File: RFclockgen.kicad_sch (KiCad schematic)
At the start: 10 parts, among them J1 Conn_01x04_Pin, J3 Conn_01x02_Pin, U2 ESP32-S3-WROOM-1, U3 AP2112K-3.3

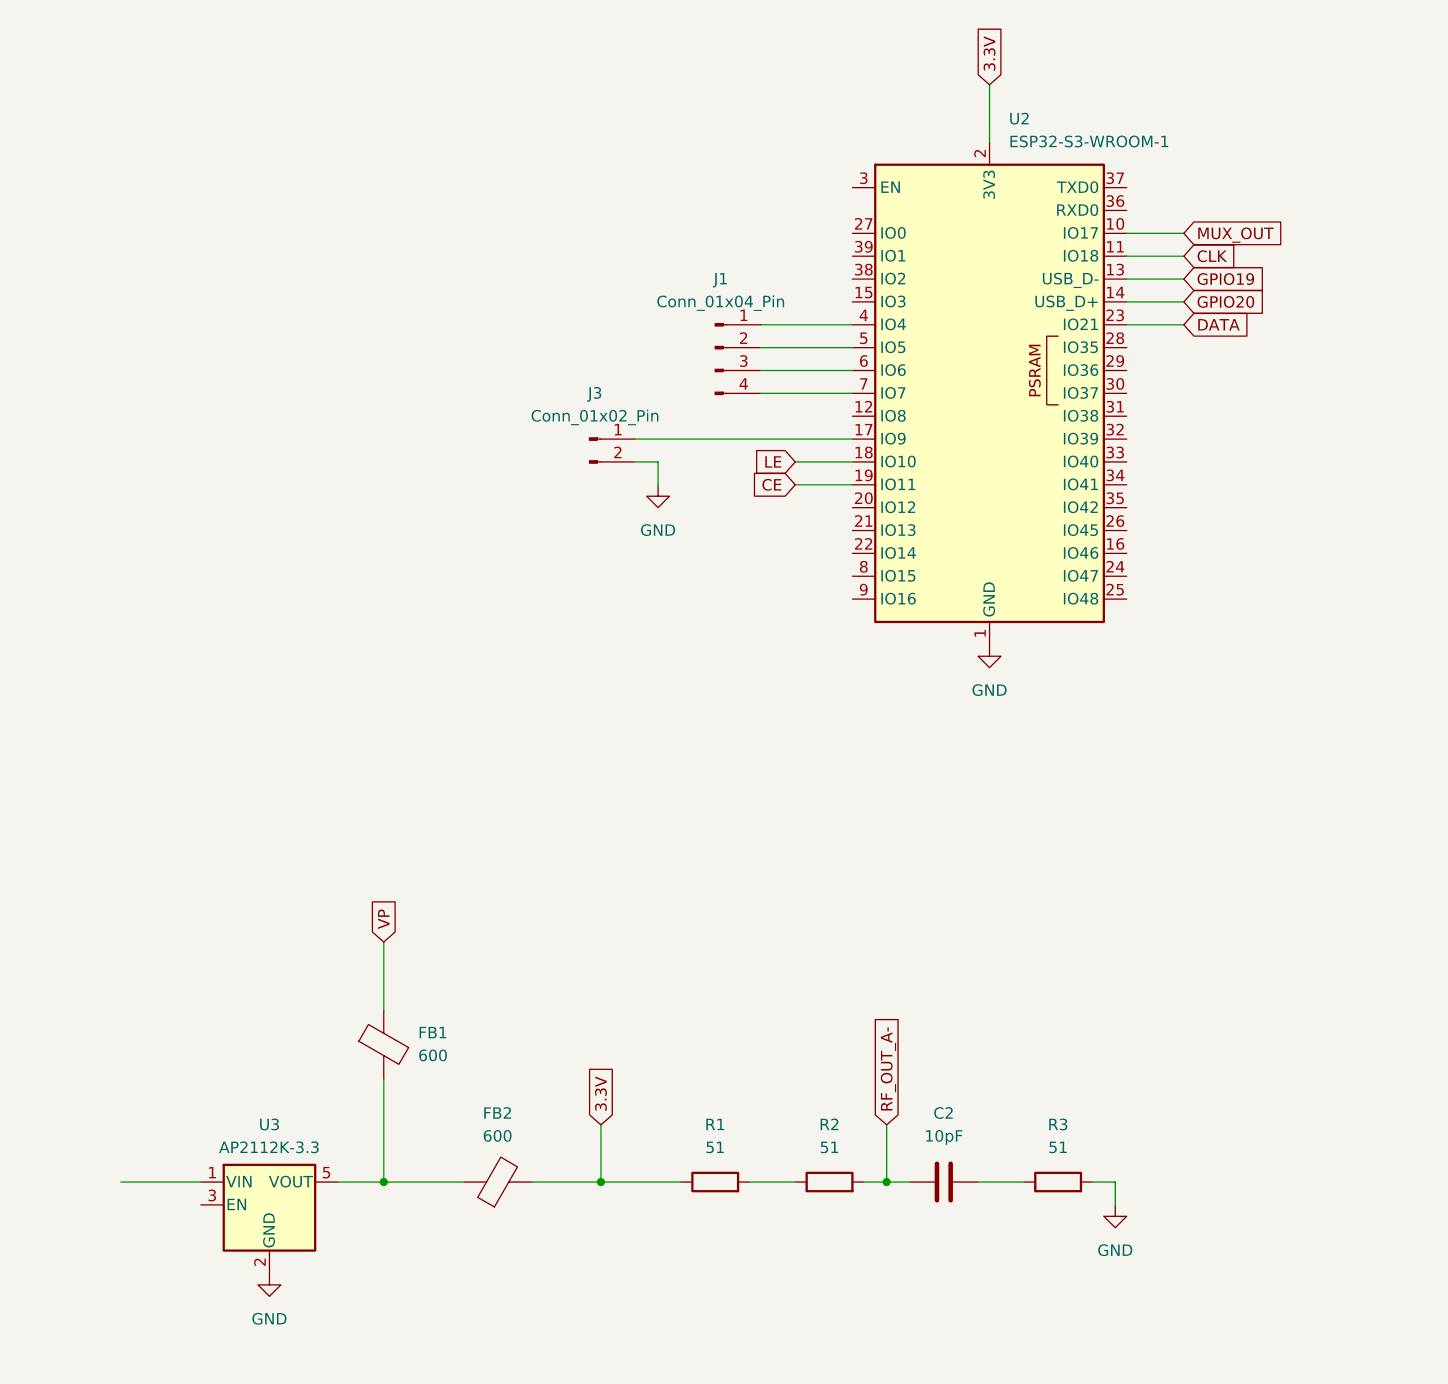
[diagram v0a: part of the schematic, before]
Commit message: updated schematic
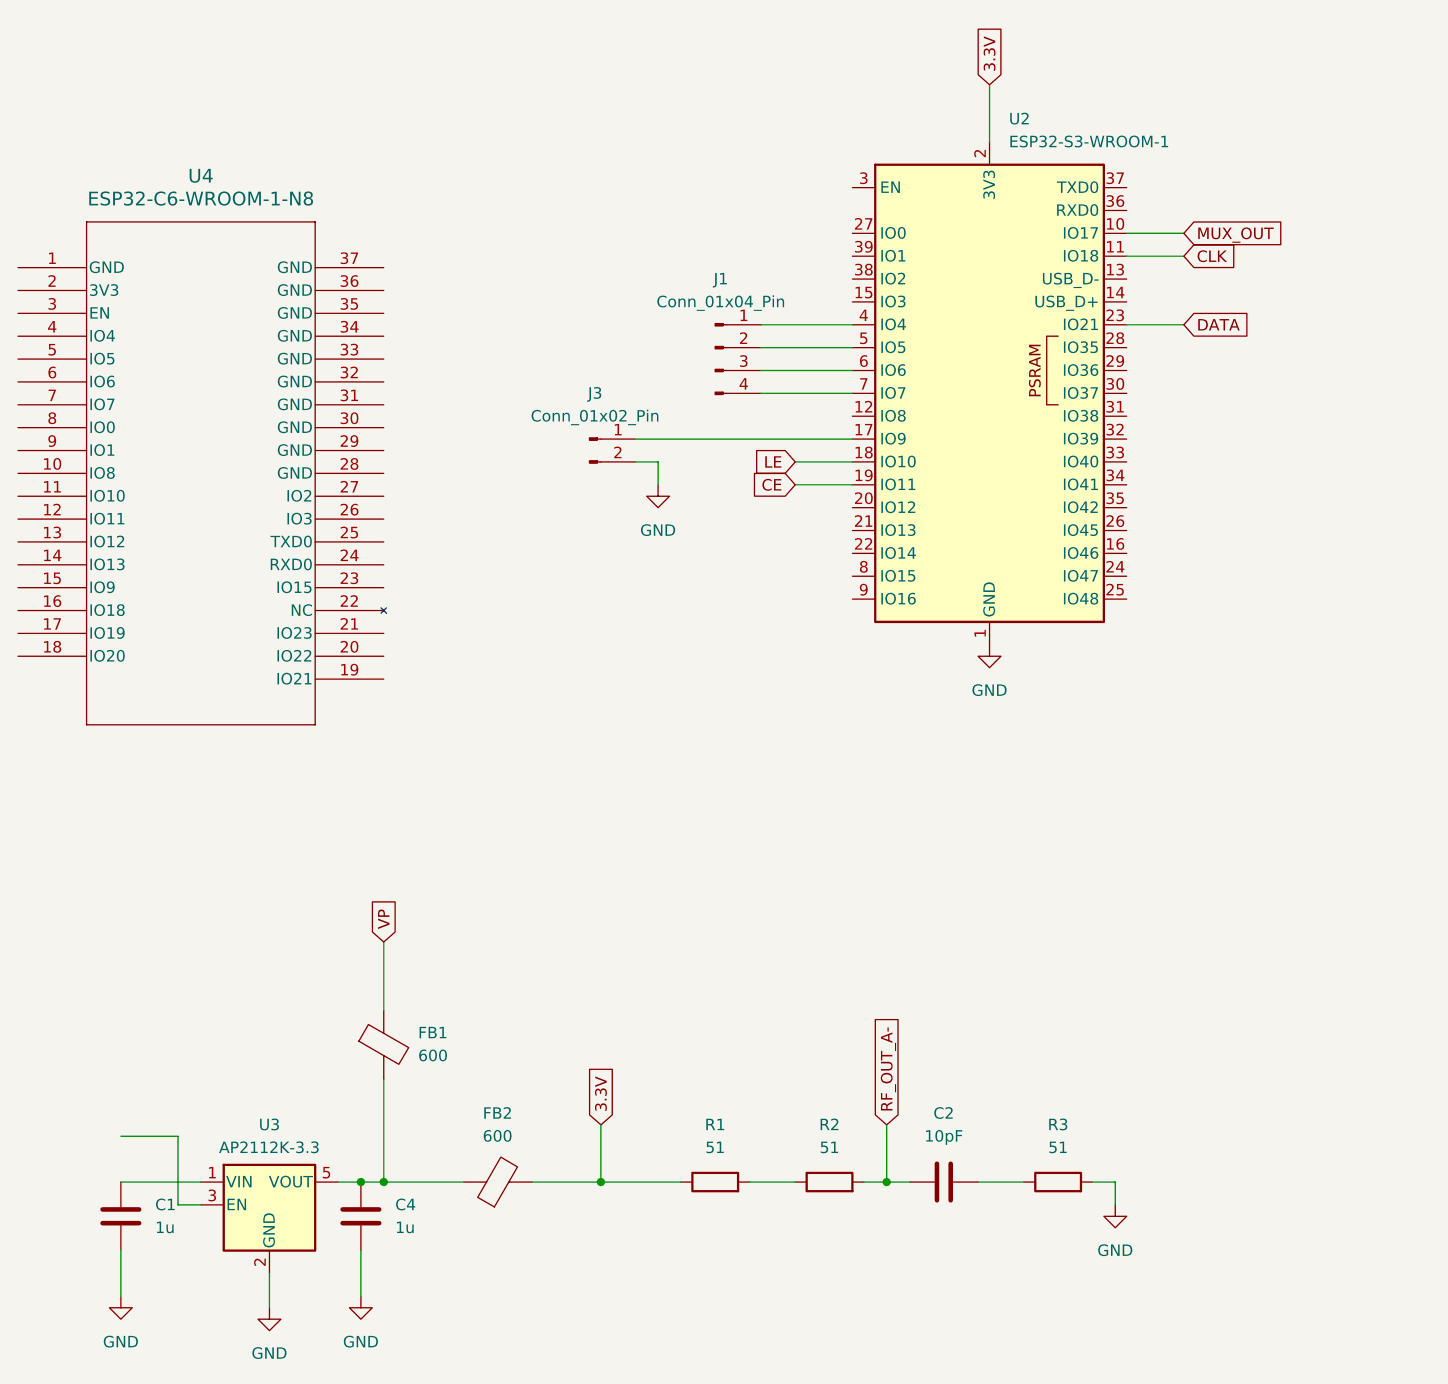
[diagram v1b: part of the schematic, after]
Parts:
- added C1, C4: 1u, symbol Device:C
- added U4: ESP32-C6-WROOM-1-N8, MOD28_ESP32-C6-WROOM-1_EXP, symbol 2026-10-07_01-33-30:ESP32-C6-WROOM-1-N8
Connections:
- net GND: now also C1.2, C4.2
- net at U3.1 (VIN): now also C1.1
- net at FB1.2, FB2.1, U3.5 (VOUT): now also C4.1
- net GPIO19: no longer names the net of U2.13 (USB_D-)
- net GPIO20: no longer names the net of U2.14 (USB_D+)
